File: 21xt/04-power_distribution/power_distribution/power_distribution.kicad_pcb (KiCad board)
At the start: 2 copper layers, 63.5 x 51.5 mm, 24 parts, among them J1 Conn_01x02, J2 Conn_01x02, J3 Conn_01x02, Q1 NMOS, Q2 NMOS, U1 LM74700, U2 XIAO-ESP32-C3-DIP, U3 LM74700, U4 INA180A1, U5 LTC2959, U6 TLV76150DCY

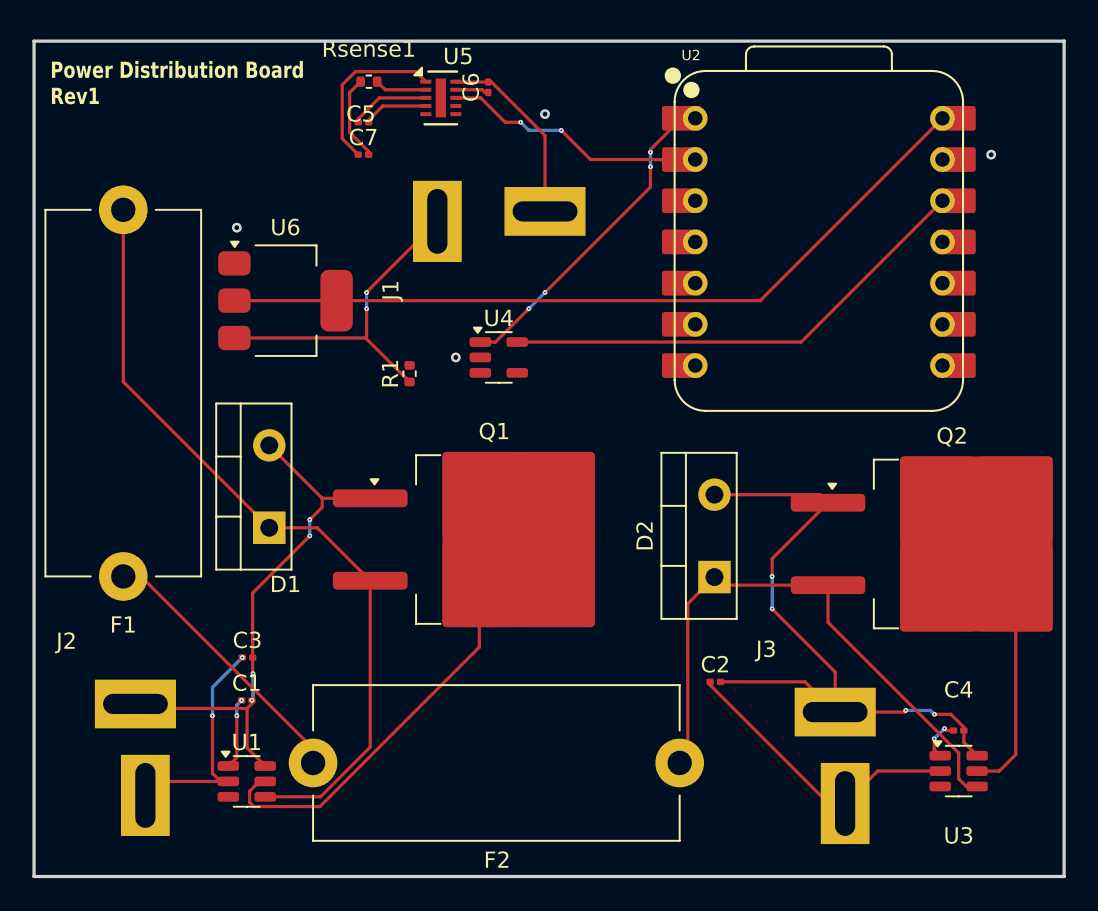
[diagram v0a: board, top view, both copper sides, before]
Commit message: redone schematic
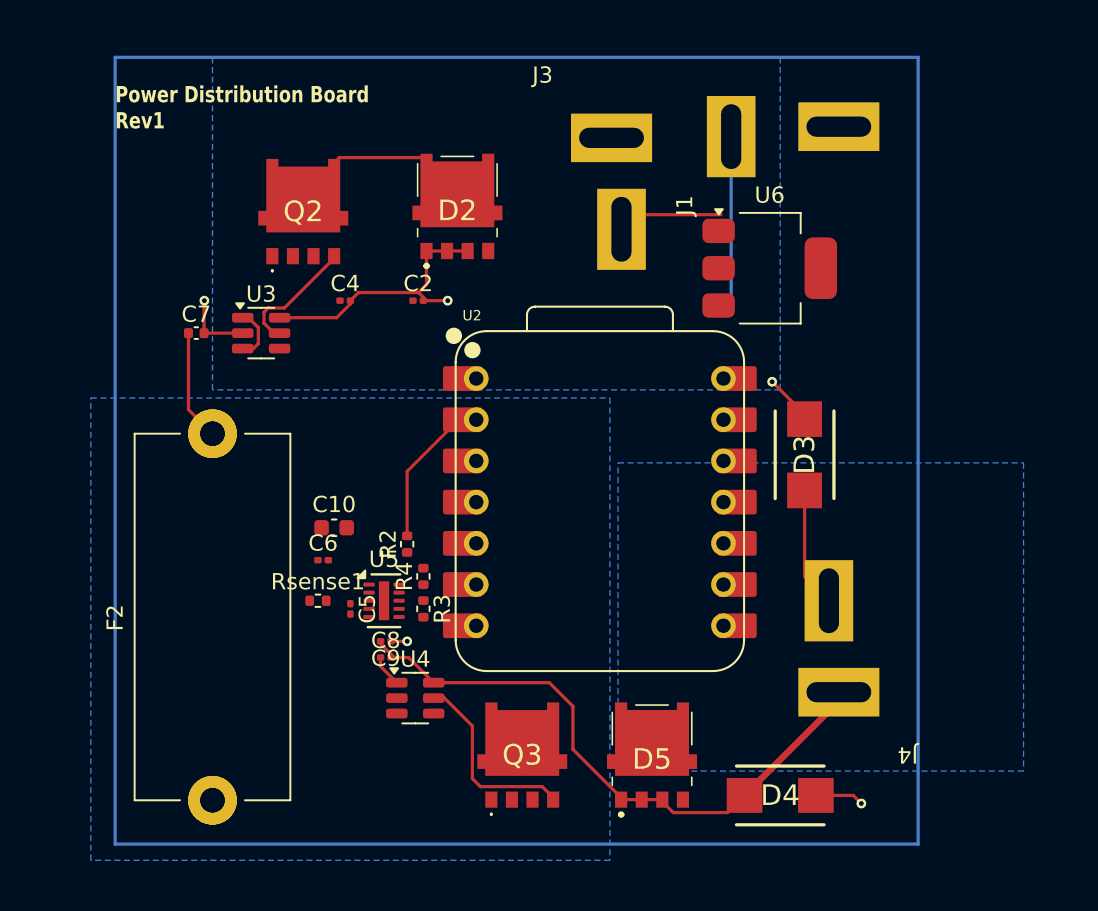
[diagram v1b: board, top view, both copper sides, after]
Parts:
- removed C1, C3: 10 uF, Capacitor_SMD:C_0201_0603Metric
- removed D1: 19A schottky, Package_TO_SOT_THT:TO-220-2_Vertical
- removed J2: Conn_01x02, 21xt_footprints:Deans Connector Male
- removed Q1: NMOS, Package_TO_SOT_SMD:TO-263-2
- removed R1: 20 mOhms, Resistor_SMD:R_0402_1005Metric
- removed U1: LM74700, Package_TO_SOT_SMD:SOT-23-6
- added C10: 100uF, Capacitor_SMD:C_0603_1608Metric, F.Cu at (117.5, 112.5)
- added C8: 10 uF, Capacitor_SMD:C_0201_0603Metric, F.Cu at (120.7, 120.5)
- added C9: 10 uF, Capacitor_SMD:C_0201_0603Metric, F.Cu at (120.7, 119.5)
- added D3: SMBJ33CA, 21xt_footprints:SMBJ33CA, F.Cu at (146.5, 108.0)
- added D4: SMBJ33CA, 21xt_footprints:SMBJ33CA, F.Cu at (145.0, 129.0)
- added D5: NRVB10100MFST1G, 21xt_footprints:NRVTS10100EMFST1G, F.Cu at (135.2, 129.3)
- added J4: Conn_01x02, 21xt_footprints:Deans Connector Male, F.Cu at (152.9, 126.0)
- added Q3: NVMFWS2D1N08XT1G, 21xt_footprints:NTMFWS1D5N08XT1G, F.Cu at (129.1, 126.5)
- added R2: 2k, Resistor_SMD:R_0402_1005Metric, F.Cu at (122.0, 113.5)
- added R3: 2k, Resistor_SMD:R_0402_1005Metric, F.Cu at (123.0, 117.5)
- added R4: 2k, Resistor_SMD:R_0402_1005Metric, F.Cu at (123.0, 115.5)
- C7: value 100 nF -> 10uF; footprint Capacitor_SMD:C_0201_0603Metric -> Capacitor_SMD:C_0402_1005Metric
- D2: value 19A schottky -> NRVB10100MFST1G; footprint Package_TO_SOT_THT:TO-220-2_Vertical -> 21xt_footprints:NRVTS10100EMFST1G
- F1: moved to B.Cu
- Q2: value NMOS -> NVMFWS2D1N08XT1G; footprint Package_TO_SOT_SMD:TO-263-2 -> 21xt_footprints:NTMFWS1D5N08XT1G
- U4: value INA180A1 -> LM74700; footprint Package_TO_SOT_SMD:SOT-23-5 -> Package_TO_SOT_SMD:SOT-23-6
- moved U3 50.8 mm to (113.0, 100.5)
- moved C4 46.2 mm to (118.2, 98.5)
- moved Q2 44.9 mm to (115.6, 93.0)
- moved J3 38.0 mm to (130.3, 85.1)
- moved Rsense1 32.2 mm to (116.5, 117.0)
- moved U5 31.2 mm to (120.6, 117.0)
- moved C6 30.9 mm to (116.8, 114.5), turned to 0 degrees
- moved C5 30.0 mm to (118.5, 117.5), turned to -90 degrees
- moved U6 29.9 mm to (144.3, 96.5)
- moved C2 29.8 mm to (122.7, 98.5)
- moved F2 28.9 mm to (110.0, 129.3), turned to 90 degrees
- moved D2 26.8 mm to (123.2, 95.5), turned to 0 degrees
- moved U4 21.6 mm to (122.5, 123.0)
- moved U2 21.0 mm to (134.0, 110.9)
- moved J1 18.9 mm to (139.6, 92.6)
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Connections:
- net Net-(U2-GPIO6/D4/SDA) renamed SDA
- net Net-(U2-GPIO7/D5/SCL) renamed SCL
- C2 pad 1: GND2 -> GND
- C4 pad 1: Net-(U3-VCAP) -> Net-(U3-EN)
- C7 pad 1: Net-(U5-V_{DD}) -> Net-(C7-Pad1)
- C7 pad 2: Net-(C7-Pad2) -> GND
- D2 pad 1: Net-(D2-K) -> Battery2
- F1 pad 1: Net-(F1-Pad1) -> Net-(C7-Pad1)
- F1 pad 2: Net-(D1-K) -> Battery1_Supply
- F2 pad 1: Net-(D2-K) -> Battery2_Supply
- F2 pad 2: Net-(F1-Pad1) -> Net-(C7-Pad1)
- J3 pad 2: GND2 -> GND
- Q2 pad 1: Battery2 -> unconnected-(Q2-S_1-Pad1)
- Q2 pad 2: Net-(Q2-G) -> unconnected-(Q2-S_2-Pad2)
- Q2 pad 3: Net-(D2-K) -> unconnected-(Q2-S_3-Pad3)
- Rsense1 pad 1: Net-(C7-Pad2) -> Net-(J1-Pin_1)
- U2 pad 1: Net-(U2-GPIO2/A0/D0) -> unconnected-(U2-GPIO2/A0/D0-Pad1)_1
- U3 pad 1: Net-(U3-VCAP) -> Net-(U3-EN)
- U3 pad 2: GND2 -> GND
- U3 pad 3: unconnected-(U3-EN-Pad3) -> Net-(U3-EN)
- U3 pad 4: Net-(D2-K) -> Battery2_Supply
- U4 pad 1: Net-(U2-GPIO2/A0/D0) -> Net-(U4-EN)
- U4 pad 3: Net-(U4-+) -> Net-(U4-EN)
- U4 pad 4: Net-(U4--) -> Battery1_Supply
- U4 pad 5: 3V3 ESP32 -> Net-(Q3-G)
- U5 pad 1: Net-(U5-V_{DD}) -> 5 LinReg
- U5 pad 8: Net-(U2-GPIO3/A1/D1) -> 3V3 ESP32
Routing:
- net Net-(D1-K): track 48.9 -> 0.00 mm
- net 5 LinReg: track 48.3 -> 0.00 mm
- net Net-(D2-K): track 36.6 -> 0.00 mm
- net 3V3 ESP32: track 29.8 -> 0.00 mm
- net Net-(Q1-G): track 24.1 -> 0.00 mm
- net Battery2: track 41.5 -> 19.9 mm, vias 4 -> 2
- net Net-(U2-GPIO2/A0/D0): track 19.5 -> 0.00 mm, vias 4 -> 0
- net GND2: track 18.2 -> 0.00 mm
- net Net-(F1-Pad1): track 17.0 -> 0.00 mm
- net GND1: track 14.5 -> 0.00 mm, vias 2 -> 0
- net Net-(Q3-G): track 0.00 -> 11.9 mm
- net Net-(U5-V_{DD}): track 10.5 -> 0.00 mm
- net Net-(J1-Pin_1): track 20.9 -> 10.8 mm, vias 2 -> 0
- net GND: track 12.6 -> 22.3 mm, vias 2 -> 3
- net Net-(U2-GPIO3/A1/D1): track 16.3 -> 8.72 mm, vias 2 -> 0
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- added copper zone on B.Cu, net Battery1_Supply
- added copper zone on B.Cu, net Battery2
- added copper zone on In1.Cu, net GND
- removed copper zone on B.Cu, net GND
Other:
- board outline removed
- copper layers 2 -> 4
